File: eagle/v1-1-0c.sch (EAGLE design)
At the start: 177 parts, among them J1 CR22A-44D-2.54DSA(70), J3 26-60-4040, J4 AUDIO_JACK_3.5MM_PTH, J5 DIN5, SW1 3PDT-AQ-SWITCH, SW2 9077-1, U10 7805, U11 74LS10N, U13 74LS04N, U14 4528N, U15 74LS86N, U16 744066N, U6 74LS165N, U7 HD61K202P-PLA1, U9 74367N

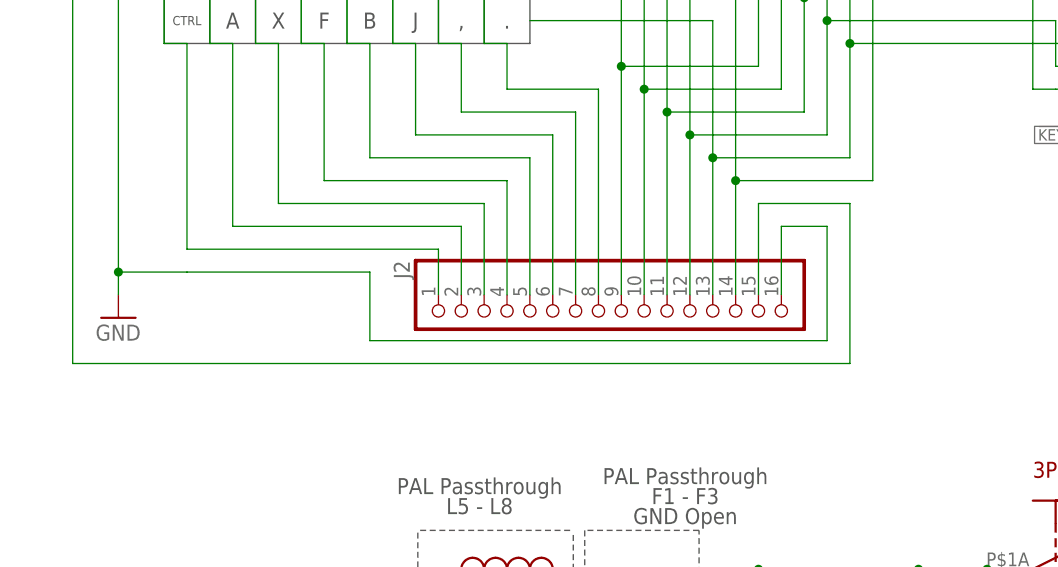
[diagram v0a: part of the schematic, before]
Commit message: Updates
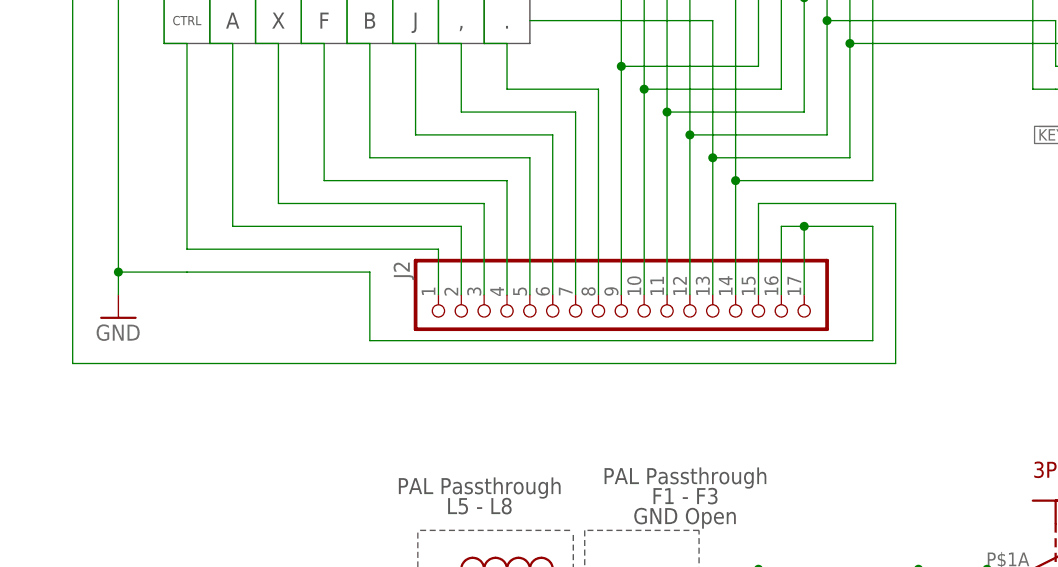
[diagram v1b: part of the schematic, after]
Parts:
- J2: device aquarius2:PINHD-1X16 -> aquarius2:PINHD-1X17
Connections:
- net GND: now also J2.17
